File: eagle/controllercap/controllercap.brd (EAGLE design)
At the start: 11.4 x 24.1 mm, 3 parts

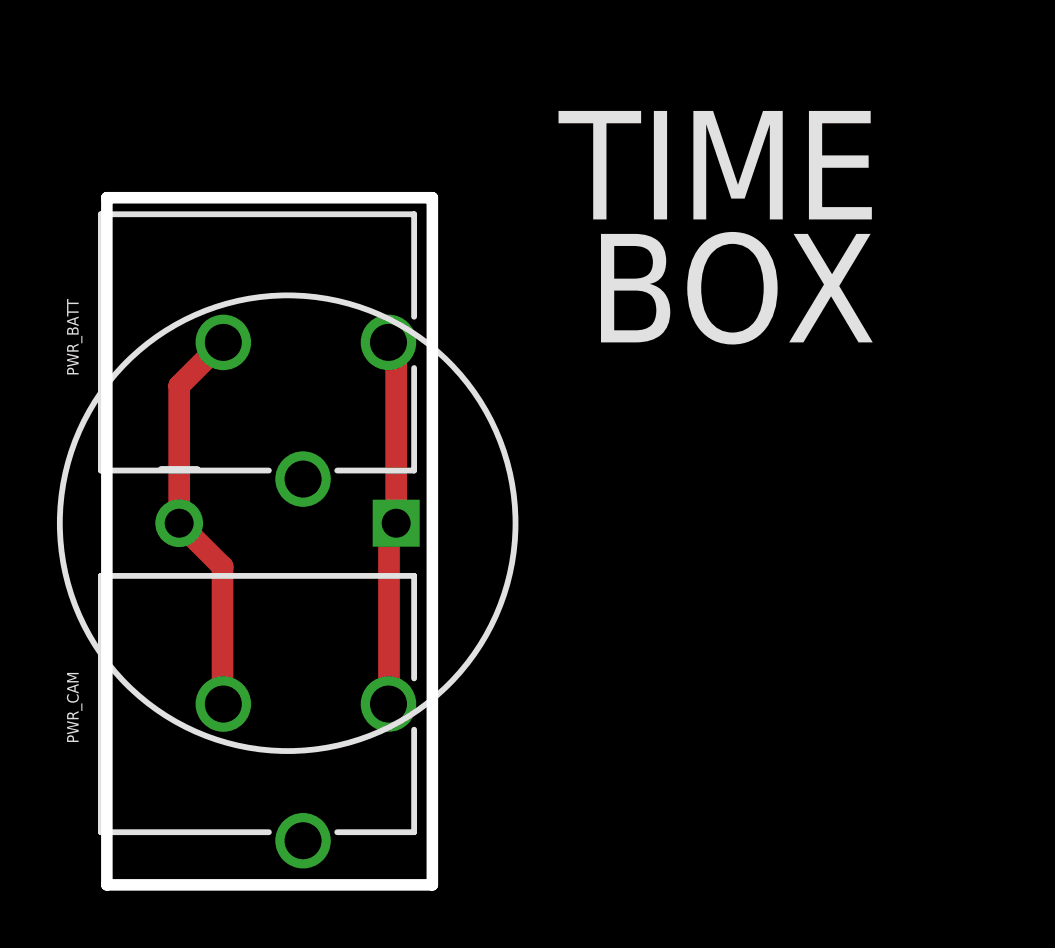
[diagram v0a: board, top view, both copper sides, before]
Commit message: minor changes
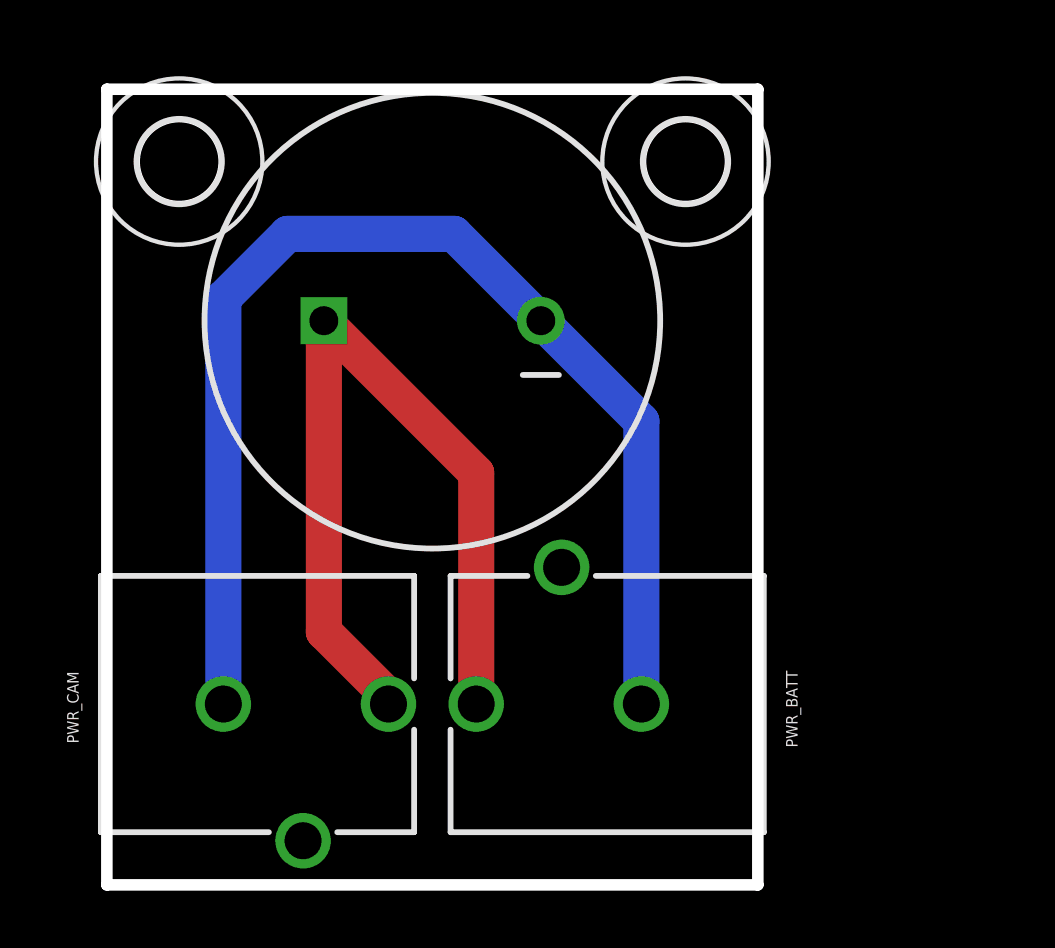
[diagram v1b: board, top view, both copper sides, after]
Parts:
- added H1, H2: MOUNT-HOLE2.8, holes:2,8
- moved PWR_BATT 33.0 mm to (26.7, 6.35), turned to 90 degrees
- moved C2 8.74 mm to (11.4, 19.8), turned to 180 degrees
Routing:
- net GNDA: track 14.0 -> 42.5 mm
- net CAM_OUT: track 12.9 -> 30.1 mm
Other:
- board size 11.4 x 24.1 mm -> 22.9 x 27.9 mm
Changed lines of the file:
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@@
 <?xml version="1.0" encoding="utf-8"?>
 <!DOCTYPE eagle SYSTEM "eagle.dtd">
-<eagle version="7.6.0">
+<eagle version="7.7.0">
 <drawing>
 <settings>
@@
 <layer number="20" name="Dimension" color="15" fill="1" visible="yes" active="yes"/>
 <layer number="21" name="tPlace" color="7" fill="1" visible="yes" active="yes"/>
-<layer number="22" name="bPlace" color="7" fill="1" visible="no" active="yes"/>
+<layer number="22" name="bPlace" color="7" fill="1" visible="yes" active="yes"/>
 <layer number="23" name="tOrigins" color="15" fill="1" visible="yes" active="yes"/>
 <layer number="24" name="bOrigins" color="15" fill="1" visible="yes" active="yes"/>
@@
 <board>
 <plain>
-<wire x1="0" y1="0" x2="11.43" y2="0" width="0.4064" layer="20"/>
-<wire x1="11.43" y1="0" x2="11.43" y2="24.13" width="0.4064" layer="20"/>
-<wire x1="11.43" y1="24.13" x2="0" y2="24.13" width="0.4064" layer="20"/>
-<wire x1="0" y1="24.13" x2="0" y2="0" width="0.4064" layer="20"/>
-<circle x="31.75" y="31.75" radius="26.518378125" width="6.4516" layer="22"/>
-<circle x="31.75" y="31.75" radius="20.517475" width="3.81" layer="22"/>
-<circle x="31.75" y="31.75" radius="16.584565625" width="2.54" layer="22"/>
-<circle x="31.75" y="31.75" radius="13.53190625" width="2.1844" layer="22"/>
-<circle x="31.75" y="31.75" radius="10.824840625" width="1.9304" layer="22"/>
-<circle x="31.75" y="31.75" radius="8.34825625" width="1.778" layer="22"/>
-<circle x="31.75" y="31.75" radius="5.97035" width="1.6764" layer="22"/>
-<circle x="31.75" y="31.75" radius="3.862553125" width="1.4224" layer="22"/>
-<circle x="31.75" y="31.75" radius="1.87513125" width="1.4224" layer="22"/>
-<text x="15.875" y="23.368" size="3.81" layer="21" ratio="15">TIME</text>
-<text x="16.891" y="19.05" size="3.81" layer="21" ratio="15">BOX</text>
+<wire x1="0" y1="0" x2="22.86" y2="0" width="0.4064" layer="20"/>
+<wire x1="22.86" y1="0" x2="22.86" y2="27.94" width="0.4064" layer="20"/>
+<wire x1="22.86" y1="27.94" x2="0" y2="27.94" width="0.4064" layer="20"/>
+<wire x1="0" y1="27.94" x2="0" y2="0" width="0.4064" layer="20"/>
+<text x="13.335" y="14.097" size="3.81" layer="22" ratio="15" rot="MR0">TIME</text>
+<text x="12.446" y="9.906" size="3.81" layer="22" ratio="15" rot="MR0">BOX</text>
 </plain>
 <attributes>
@@
 </autorouter>
 <elements>
-<element name="PWR_BATT" library="SparkFun-Connectors" package="POWER_JACK_PTH_BREAD" value="" x="-3.81" y="19.05" smashed="yes" rot="R270">
-<attribute name="PROD_ID" value="PRT-10811" x="-3.81" y="19.05" size="1.778" layer="27" rot="R270" display="off"/>
-<attribute name="NAME" x="-1.397" y="20.574" size="0.4064" layer="25" rot="R270"/>
-<attribute name="VALUE" x="0.25" y="22.86" size="0.4064" layer="27" rot="R270"/>
+<element name="PWR_BATT" library="SparkFun-Connectors" package="POWER_JACK_PTH_BREAD" value="" x="26.67" y="6.35" smashed="yes" rot="R90">
+<attribute name="PROD_ID" value="PRT-10811" x="26.67" y="6.35" size="1.778" layer="27" rot="R90" display="off"/>
+<attribute name="NAME" x="24.257" y="4.826" size="0.4064" layer="25" rot="R90"/>
+<attribute name="VALUE" x="22.61" y="2.54" size="0.4064" layer="27" rot="R90"/>
 </element>
 <element name="PWR_CAM" library="SparkFun-Connectors" package="POWER_JACK_PTH_BREAD" value="" x="-3.81" y="6.35" smashed="yes" rot="R270">
@@
 <attribute name="VALUE" x="0.25" y="10.16" size="0.4064" layer="27" rot="R270"/>
 </element>
-<element name="C2" library="SparkFun-Passives" package="CPOL-RADIAL-1000UF-63V" value="4700uF" x="6.35" y="12.7" smashed="yes">
-<attribute name="VALUE" x="4.318" y="12.192" size="0.8128" layer="27"/>
+<element name="C2" library="SparkFun-Passives" package="CPOL-RADIAL-1000UF-63V" value="4700uF" x="11.43" y="19.812" smashed="yes" rot="R180">
+<attribute name="VALUE" x="13.462" y="20.32" size="0.8128" layer="27" rot="R180"/>
 </element>
+<element name="H1" library="holes" package="2,8" value="MOUNT-HOLE2.8" x="2.54" y="25.4"/>
+<element name="H2" library="holes" package="2,8" value="MOUNT-HOLE2.8" x="20.32" y="25.4"/>
 </elements>
 <signals>
@@
 <contactref element="C2" pad="1"/>
 <contactref element="PWR_BATT" pad="PWR"/>
-<wire x1="10.16" y1="18.796" x2="10.16" y2="12.7" width="0.762" layer="1"/>
-<wire x1="9.906" y1="19.05" x2="10.16" y2="18.796" width="0.762" layer="1"/>
-<wire x1="9.906" y1="19.05" x2="9.89" y2="19.05" width="0.762" layer="1"/>
-<wire x1="9.906" y1="12.446" x2="9.906" y2="6.35" width="0.762" layer="1"/>
-<wire x1="9.906" y1="6.35" x2="9.89" y2="6.35" width="0.762" layer="1"/>
-<wire x1="9.906" y1="12.446" x2="10.16" y2="12.7" width="0.762" layer="1"/>
+<wire x1="12.97" y1="6.35" x2="12.97" y2="14.462" width="1.27" layer="1"/>
+<wire x1="12.97" y1="14.462" x2="7.62" y2="19.812" width="1.27" layer="1"/>
+<wire x1="9.89" y1="6.35" x2="9.89" y2="6.62" width="1.27" layer="1"/>
+<wire x1="9.89" y1="6.62" x2="7.62" y2="8.89" width="1.27" layer="1"/>
+<wire x1="7.62" y1="8.89" x2="7.62" y2="19.812" width="1.27" layer="1"/>
 </signal>
 <signal name="GNDA" class="1">
@@
 <contactref element="PWR_CAM" pad="GND"/>
 <contactref element="C2" pad="2"/>
-<wire x1="2.54" y1="17.526" x2="2.54" y2="12.7" width="0.762" layer="1"/>
-<wire x1="4.064" y1="19.05" x2="2.54" y2="17.526" width="0.762" layer="1"/>
-<wire x1="4.064" y1="19.05" x2="4.09" y2="19.05" width="0.762" layer="1"/>
-<wire x1="4.064" y1="11.176" x2="4.064" y2="6.35" width="0.762" layer="1"/>
-<wire x1="2.54" y1="12.7" x2="4.064" y2="11.176" width="0.762" layer="1"/>
-<wire x1="4.064" y1="6.35" x2="4.09" y2="6.35" width="0.762" layer="1"/>
+<wire x1="18.77" y1="6.35" x2="18.77" y2="16.282" width="1.27" layer="16"/>
+<wire x1="18.77" y1="16.282" x2="15.24" y2="19.812" width="1.27" layer="16"/>
+<wire x1="4.09" y1="6.35" x2="4.09" y2="20.6" width="1.27" layer="16"/>
+<wire x1="4.09" y1="20.6" x2="6.35" y2="22.86" width="1.27" layer="16"/>
+<wire x1="6.35" y1="22.86" x2="12.192" y2="22.86" width="1.27" layer="16"/>
+<wire x1="12.192" y1="22.86" x2="15.24" y2="19.812" width="1.27" layer="16"/>
 </signal>
 </signals>
